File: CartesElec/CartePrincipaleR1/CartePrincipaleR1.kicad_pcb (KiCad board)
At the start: 2 copper layers, 100 x 100 mm, 27 parts, among them U1 LT1129-3.3_SOT223

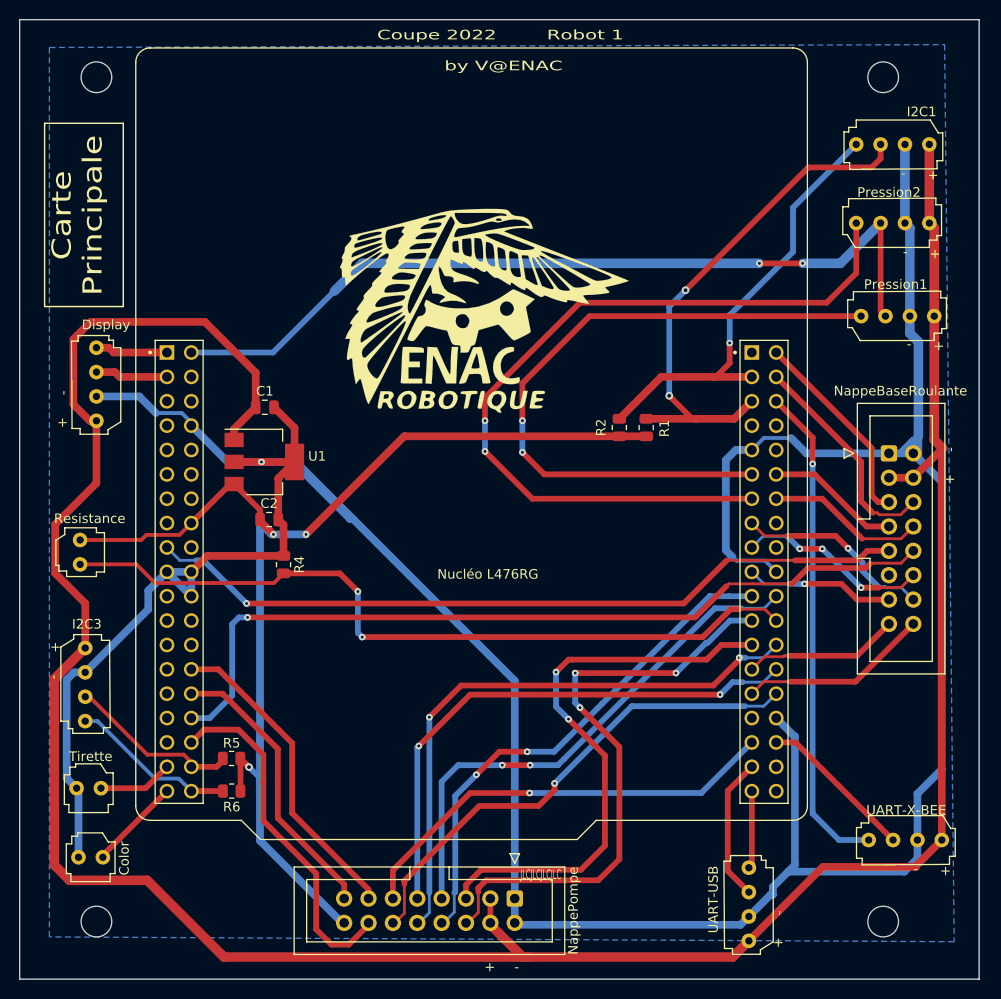
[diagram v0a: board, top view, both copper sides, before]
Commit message: Modif dernière minute
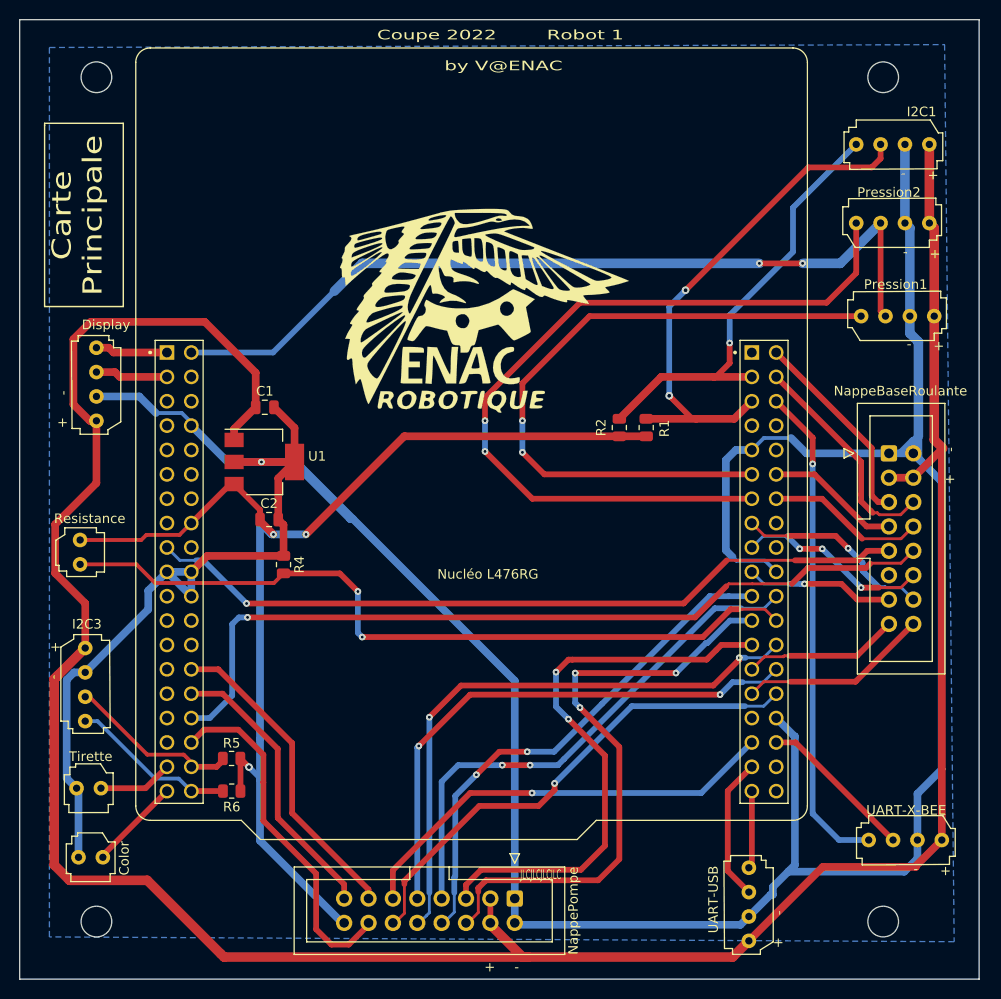
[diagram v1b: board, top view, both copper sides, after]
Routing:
- net SDA_I2C3: track 18.3 -> 17.7 mm
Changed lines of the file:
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@@
   (segment (start 78.0125 115.4) (end 78.0125 112.0125) (width 0.6) (layer "F.Cu") (net 3))
   (segment (start 117.5 78.425) (end 95.175 78.425) (width 0.8) (layer "F.Cu") (net 3))
-  (segment (start 117.5875 78.3375) (end 117.5 78.425) (width 0.4) (layer "F.Cu") (net 3))
   (segment (start 67.67 89.23) (end 61.3 89.23) (width 0.4) (layer "F.Cu") (net 3))
   (segment (start 95.175 78.425) (end 95.075 78.425) (width 0.8) (layer "F.Cu") (net 3))
@@
   (segment (start 68.12 115.1) (end 63.47 115.1) (width 0.6) (layer "F.Cu") (net 5))
   (segment (start 68.3 111.6) (end 62.27 105.57) (width 0.4) (layer "F.Cu") (net 6))
-  (segment (start 72.89 112.87) (end 72.89 112.39) (width 0.4) (layer "F.Cu") (net 6))
   (segment (start 72.1 111.6) (end 68.3 111.6) (width 0.4) (layer "F.Cu") (net 6))
   (segment (start 76.175 112.225) (end 76.175 112) (width 0.6) (layer "F.Cu") (net 6))
@@
   (segment (start 75.53 112.87) (end 76.175 112.225) (width 0.6) (layer "F.Cu") (net 6))
   (segment (start 75.53 112.87) (end 72.89 112.87) (width 0.6) (layer "F.Cu") (net 6))
-  (segment (start 73.02 113) (end 72.89 112.87) (width 0.6) (layer "F.Cu") (net 6))
   (segment (start 62.27 105.57) (end 61.832 105.57) (width 0.4) (layer "F.Cu") (net 6))
   (segment (start 72.9 115.4) (end 72.89 115.41) (width 0.6) (layer "F.Cu") (net 7))
@@
   (segment (start 137.84 82.39) (end 133.85 82.39) (width 0.6) (layer "F.Cu") (net 14))
   (segment (start 133.85 84.93) (end 138.63 84.93) (width 0.6) (layer "F.Cu") (net 15))
-  (segment (start 142.860489 89.160489) (end 142.8 89.1) (width 0.3) (layer "F.Cu") (net 15))
   (segment (start 148.14 87.82) (end 146.86 89.1) (width 0.3) (layer "F.Cu") (net 15))
   (segment (start 146.86 89.1) (end 142.8 89.1) (width 0.3) (layer "F.Cu") (net 15))
@@
   (segment (start 117.5 122.5) (end 115.3 124.7) (width 0.6) (layer "F.Cu") (net 25))
   (segment (start 102.8 128.06) (end 102.8 125.9) (width 0.3) (layer "F.Cu") (net 25))
-  (segment (start 112.9 103.1) (end 112.8 103.1) (width 0.6) (layer "F.Cu") (net 25))
   (segment (start 113.4 106.7) (end 117.5 110.8) (width 0.6) (layer "F.Cu") (net 25))
   (segment (start 102.8 125.5) (end 103.6 124.7) (width 0.6) (layer "F.Cu") (net 25))
@@
   (via (at 107.9 111.3) (size 0.7) (drill 0.3) (layers "F.Cu" "B.Cu") (net 27))
   (via (at 102.6 113.7) (size 0.7) (drill 0.3) (layers "F.Cu" "B.Cu") (net 27))
+  (segment (start 100.4 115.9) (end 100.4 124.3) (width 0.6) (layer "B.Cu") (net 27))
   (segment (start 102.6 113.7) (end 100.4 115.9) (width 0.6) (layer "B.Cu") (net 27))
   (segment (start 131.31 95.09) (end 128.91 95.09) (width 0.6) (layer "B.Cu") (net 27))
+  (segment (start 100.4 124.3) (end 100.3 124.4) (width 0.6) (layer "B.Cu") (net 27))
   (segment (start 115.7 106.3) (end 110.7 111.3) (width 0.6) (layer "B.Cu") (net 27))
   (segment (start 126.91 95.09) (end 115.7 106.3) (width 0.6) (layer "B.Cu") (net 27))
   (segment (start 100.3 128.02) (end 100.3 126) (width 0.3) (layer "B.Cu") (net 27))
+  (segment (start 100.3 124.4) (end 100.3 126) (width 0.6) (layer "B.Cu") (net 27))
   (segment (start 110.7 111.3) (end 107.9 111.3) (width 0.6) (layer "B.Cu") (net 27))
-  (segment (start 100.4 115.9) (end 100.4 125.9) (width 0.6) (layer "B.Cu") (net 27))
-  (segment (start 100.4 125.9) (end 100.3 126) (width 0.6) (layer "B.Cu") (net 27))
   (segment (start 128.91 95.09) (end 126.96 95.09) (width 0.6) (layer "B.Cu") (net 27))
   (segment (start 126.96 95.09) (end 126.91 95.09) (width 0.6) (layer "B.Cu") (net 27))
@@
   (segment (start 130.6 106.55) (end 118.8 106.55) (width 0.6) (layer "B.Cu") (net 30))
   (segment (start 118.8 106.55) (end 110.75 114.6) (width 0.6) (layer "B.Cu") (net 30))
-  (segment (start 101.95 115.6) (end 108.15 115.6) (width 0.6) (layer "F.Cu") (net 31))
   (segment (start 101.95 115.6) (end 93.9 123.65) (width 0.6) (layer "F.Cu") (net 31))
   (segment (start 93.9 123.65) (end 93.9 126.8) (width 0.6) (layer "F.Cu") (net 31))
-  (via (at 108.15 115.6) (size 0.7) (drill 0.3) (layers "F.Cu" "B.Cu") (net 31))
-  (segment (start 108.15 115.6) (end 126.04 115.6) (width 0.6) (layer "B.Cu") (net 31))
-  (segment (start 108.15 115.6) (end 108.1 115.6) (width 0.6) (layer "B.Cu") (net 31))
-  (segment (start 131.31 110.33) (end 126.04 115.6) (width 0.6) (layer "B.Cu") (net 31))
+  (segment (start 108.4 115.6) (end 101.95 115.6) (width 0.6) (layer "F.Cu") (net 31))
+  (via (at 108.4 115.6) (size 0.7) (drill 0.3) (layers "F.Cu" "B.Cu") (net 31))
+  (segment (start 126.04 115.6) (end 131.31 110.33) (width 0.6) (layer "B.Cu") (net 31))
+  (segment (start 108.4 115.6) (end 126.04 115.6) (width 0.6) (layer "B.Cu") (net 31))
   (segment (start 91.36 125.66) (end 91.36 126.8) (width 0.6) (layer "F.Cu") (net 32))
   (segment (start 83.4 110.4) (end 83.4 117.7) (width 0.6) (layer "F.Cu") (net 32))
